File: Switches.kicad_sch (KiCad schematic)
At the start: 30 parts, among them SW10 SW_SPST, SW11 PEC11R, SW12 PEC11R, SW13 PEC11R, SW2 SW_SPST, SW3 SW_SPST, SW4 SW_SPST, SW5 SW_SPST, SW6 SW_SPST, SW7 SW_SPST, SW8 SW_SPST, SW9 SW_SPST

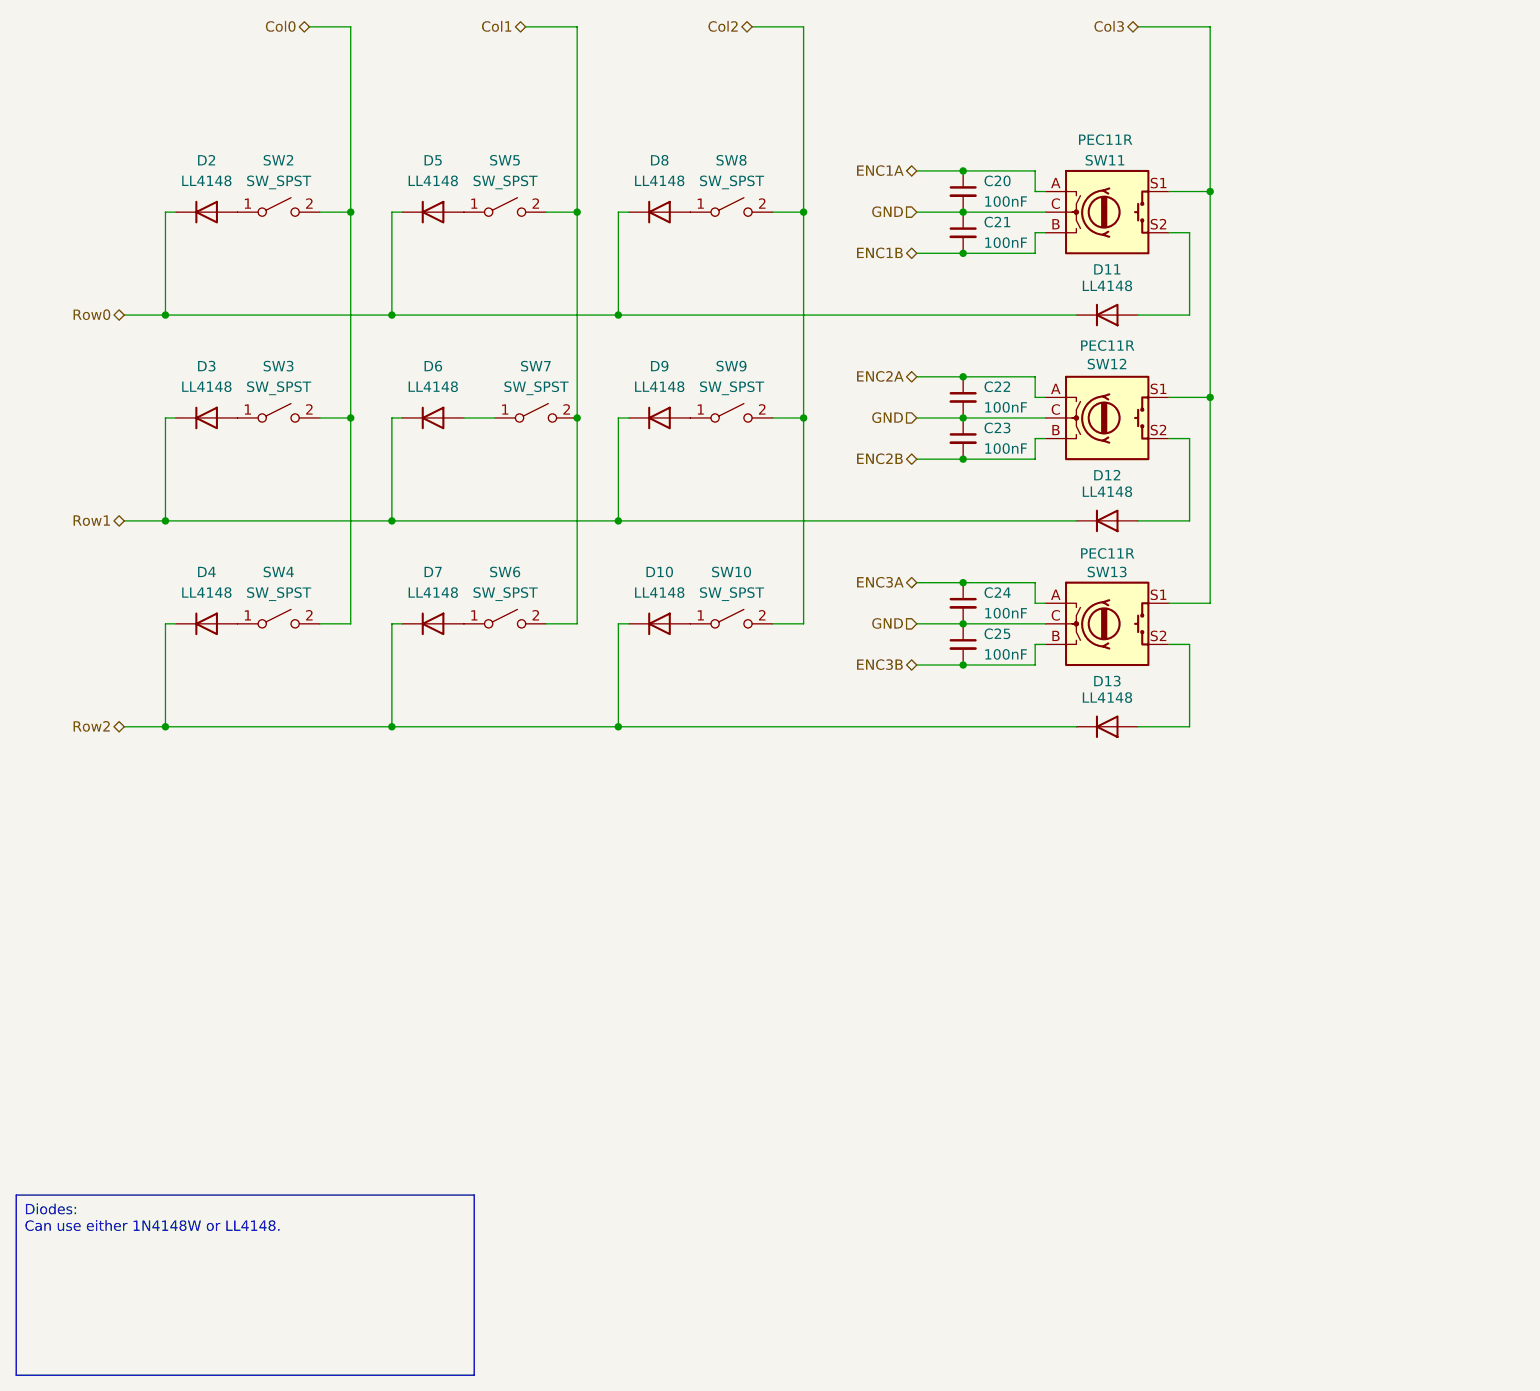
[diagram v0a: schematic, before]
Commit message: Refactor, cleanup, add todo list, update metadata on BOM
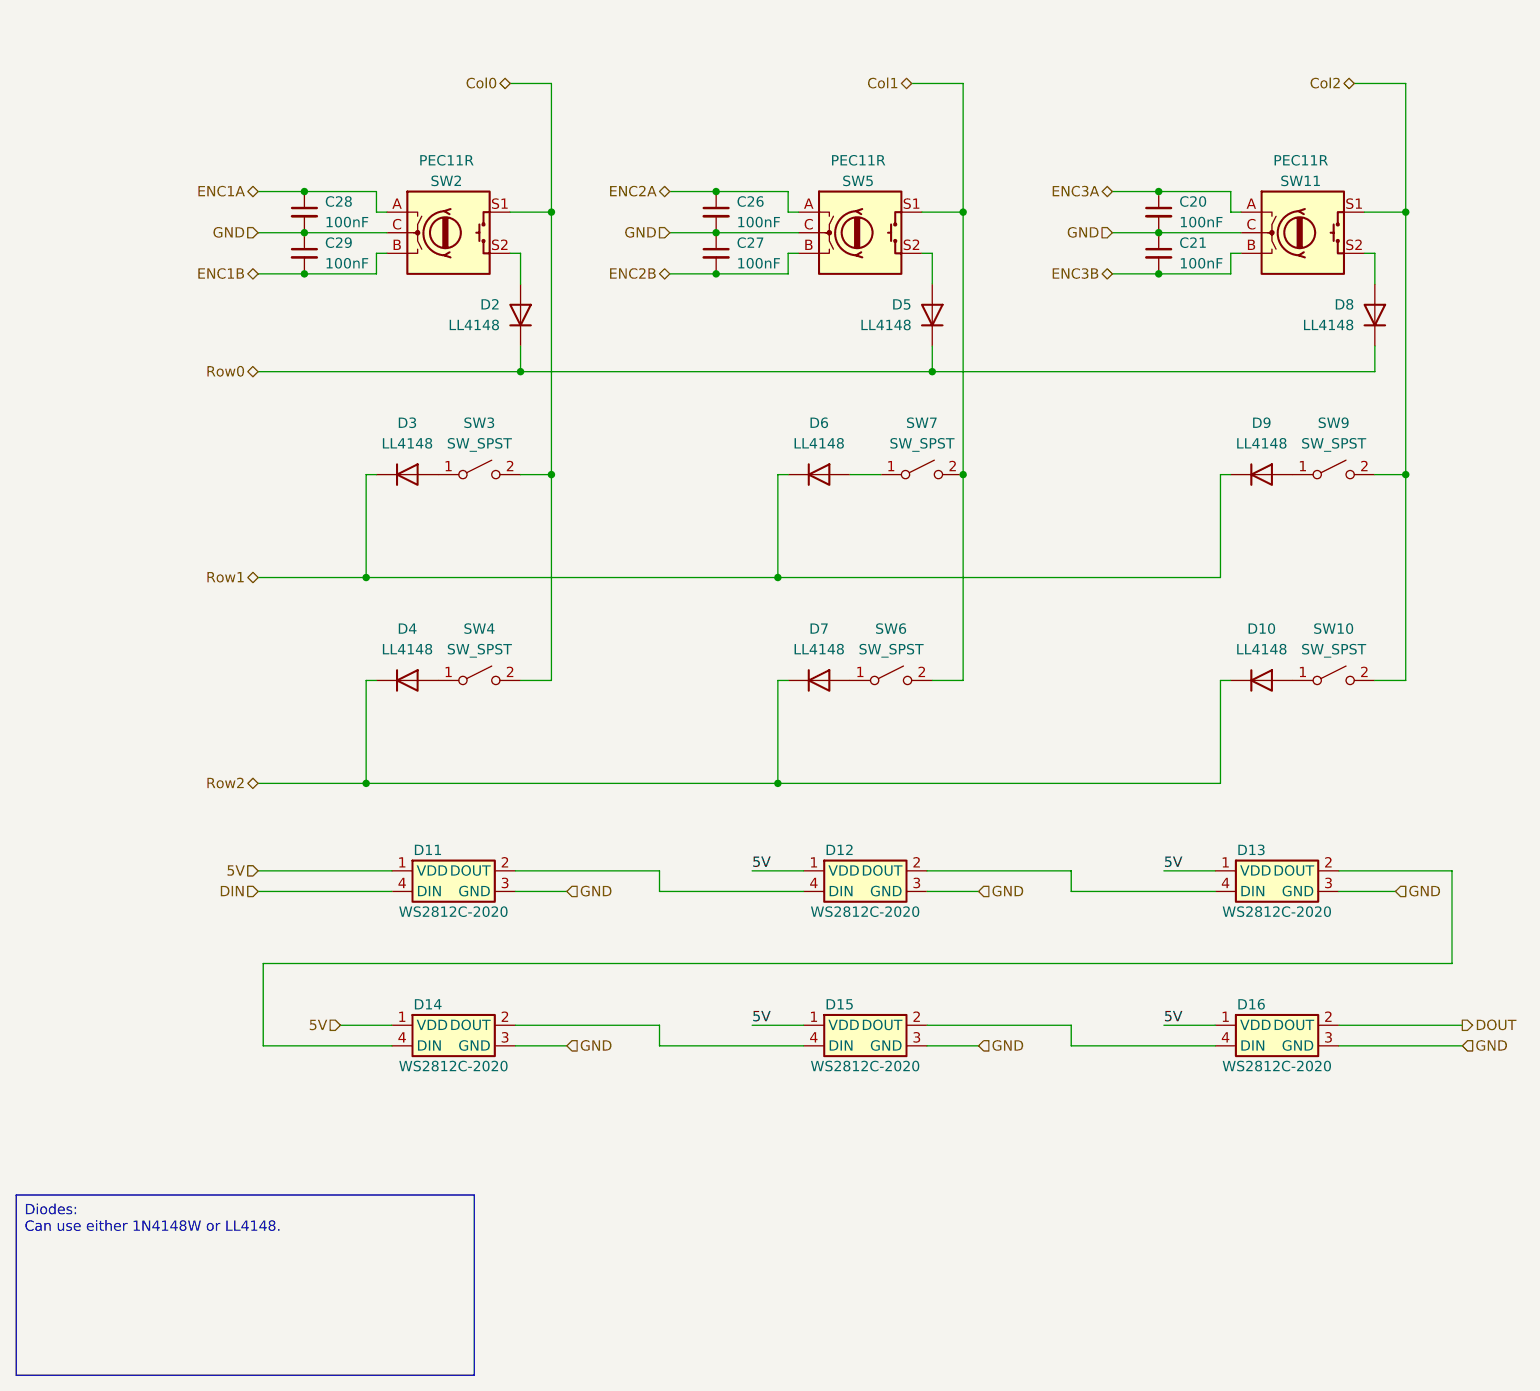
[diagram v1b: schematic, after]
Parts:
- removed C22, C23, C24, C25: 100nF, Capacitor_SMD:C_0402_1005Metric, symbol Device:C_Small
- removed D11, D12, D13: LL4148, Diode_SMD:D_MiniMELF, symbol Diode:LL4148
- removed SW12, SW13: PEC11R, Mad_Footprints:RotaryEncoder_Bourns_Vertical_PEC12R-3x17F-Sxxxx, symbol Device:RotaryEncoder_Switch
- removed SW2, SW5, SW8: SW_SPST, Mad_Footprints:SW_Hotswap_Kailh_MX_1.00u, symbol Switch:SW_SPST
- added C26, C27, C28, C29: 100nF, Capacitor_SMD:C_0402_1005Metric, symbol Device:C_Small
- added D11, D12, D13, D14, D15, D16: WS2812C-2020, Mad_Footprints:SK6812_mini_e, symbol Mad_Symbols:SK6812_Mini_E
- added SW2, SW5: PEC11R, Mad_Footprints:RotaryEncoder_Bourns_Vertical_PEC12R-3x17F-Sxxxx, symbol Device:RotaryEncoder_Switch
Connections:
- net Col3 is gone; now on net Col2: SW11.S1
- net Col0: now also SW2.S1
- net Col1: now also SW5.S1
- net ENC1A: now also C28.1, SW2.A; no longer C20.1, SW11.A
- net ENC1B: now also C29.2, SW2.B; no longer C21.2, SW11.B
- net ENC2A: now also C26.1, SW5.A
- net ENC2B: now also C27.2, SW5.B
- net ENC3A: now also C20.1, SW11.A
- net ENC3B: now also C21.2, SW11.B
- net GND: now also C26.2, C27.1, C28.2, C29.1, D11.3 (GND), D12.3 (GND), D13.3 (GND), D14.3 (GND), D15.3 (GND), D16.3 (GND), SW2.C, SW5.C
- net at D2.2 (A): now also SW2.S2
- net at D5.2 (A): now also SW5.S2
- net at SW11.S2: now also D8.2 (A)
- new net: D11.2 (DOUT), D12.4 (DIN)
- new net: D15.2 (DOUT), D16.4 (DIN)
- new net: D12.2 (DOUT), D13.4 (DIN)
- new net: D14.2 (DOUT), D15.4 (DIN)
- new net: D13.2 (DOUT), D14.4 (DIN)
- new net 5V: D11.1 (VDD), D12.1 (VDD), D13.1 (VDD), D14.1 (VDD), D15.1 (VDD), D16.1 (VDD)
- new net DIN: D11.4 (DIN)
- new net DOUT: D16.2 (DOUT)
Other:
- moved on the sheet: C20, C21, D10, D3, D4, D6, D7, D8, D9, SW10, SW11, SW3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
